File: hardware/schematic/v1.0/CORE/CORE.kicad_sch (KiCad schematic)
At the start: 80 parts, among them J1 Conn_01x06_Socket, J10 USB_C_Receptacle_USB2.0_16P, J11 Conn_01x06_Socket, J12 Conn_Coaxial, J13 Conn_01x04_Socket, J14 Conn_01x03_Socket, J15 Conn_01x05_Socket, J16 Conn_01x04_Socket, J2 Conn_Coaxial, J26 Conn_01x04_Socket, J3 Conn_Coaxial, J4 Conn_Coaxial, J5 Conn_Coaxial, J6 Conn_Coaxial, J7 Conn_Coaxial, J8 Conn_Coaxial, J9 Conn_Coaxial, M1 ZYNQ7010&7020, U1 TXS02612RTWR, U2 TPS78633, U3 SD_Card, U5 AMS1117-1.8, U6 CH340E

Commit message: sch update
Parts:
- added RGB TFTLCD1: RGBLCD, AD:FPC-TOP40, symbol Counter:FPC-40
- added U7: FPC-6P, symbol Counter:FPC-6P
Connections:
- net +3.3V: now also RGB TFTLCD1.4, U7.2
- net GND: now also RGB TFTLCD1.29, RGB TFTLCD1.3, RGB TFTLCD1.36, RGB TFTLCD1.A, RGB TFTLCD1.B, U7.3, U7.7 (SH), U7.8 (SH)
- net I2C_SCL renamed PS_I2C_SCL
- net I2C_SDA renamed PS_I2C_SDA
- net SPI1_MISO renamed PS_SPI1_MISO
- net SPI1_MOSI renamed PS_SPI1_MOSI
- net SPI1_SCLK renamed PS_SPI1_SCLK
- net SPI1_SS0 renamed PS_SPI1_SS0
- new net CTP_INT: U7.4
- new net CTP_RST: U7.1
- new net CTP_SCL: U7.6
- new net CTP_SDA: U7.5
- new net LCD_B0: RGB TFTLCD1.21
- new net LCD_B1: RGB TFTLCD1.22
- new net LCD_B2: RGB TFTLCD1.23
- new net LCD_B3: RGB TFTLCD1.24
- new net LCD_B4: RGB TFTLCD1.25
- new net LCD_B5: RGB TFTLCD1.26
- new net LCD_B6: RGB TFTLCD1.27
- new net LCD_B7: RGB TFTLCD1.28
- new net LCD_CLK: RGB TFTLCD1.30
- new net LCD_DE: RGB TFTLCD1.34
- new net LCD_DISP: RGB TFTLCD1.31
- new net LCD_G0: RGB TFTLCD1.13
- new net LCD_G1: RGB TFTLCD1.14
- new net LCD_G2: RGB TFTLCD1.15
- new net LCD_G3: RGB TFTLCD1.16
- new net LCD_G4: RGB TFTLCD1.17
- new net LCD_G5: RGB TFTLCD1.18
- new net LCD_G6: RGB TFTLCD1.19
- new net LCD_G7: RGB TFTLCD1.20
- new net LCD_HSYNC: RGB TFTLCD1.32
- new net LCD_R0: RGB TFTLCD1.5
- new net LCD_R1: RGB TFTLCD1.6
- new net LCD_R2: RGB TFTLCD1.7
- new net LCD_R3: RGB TFTLCD1.8
- new net LCD_R4: RGB TFTLCD1.9
- new net LCD_R5: RGB TFTLCD1.10
- new net LCD_R6: RGB TFTLCD1.11
- new net LCD_R7: RGB TFTLCD1.12
- new net LCD_VSYNC: RGB TFTLCD1.33
- no-connect marks 23 -> 28
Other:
- note added: "RGB888"
- moved on the sheet: J1, J11

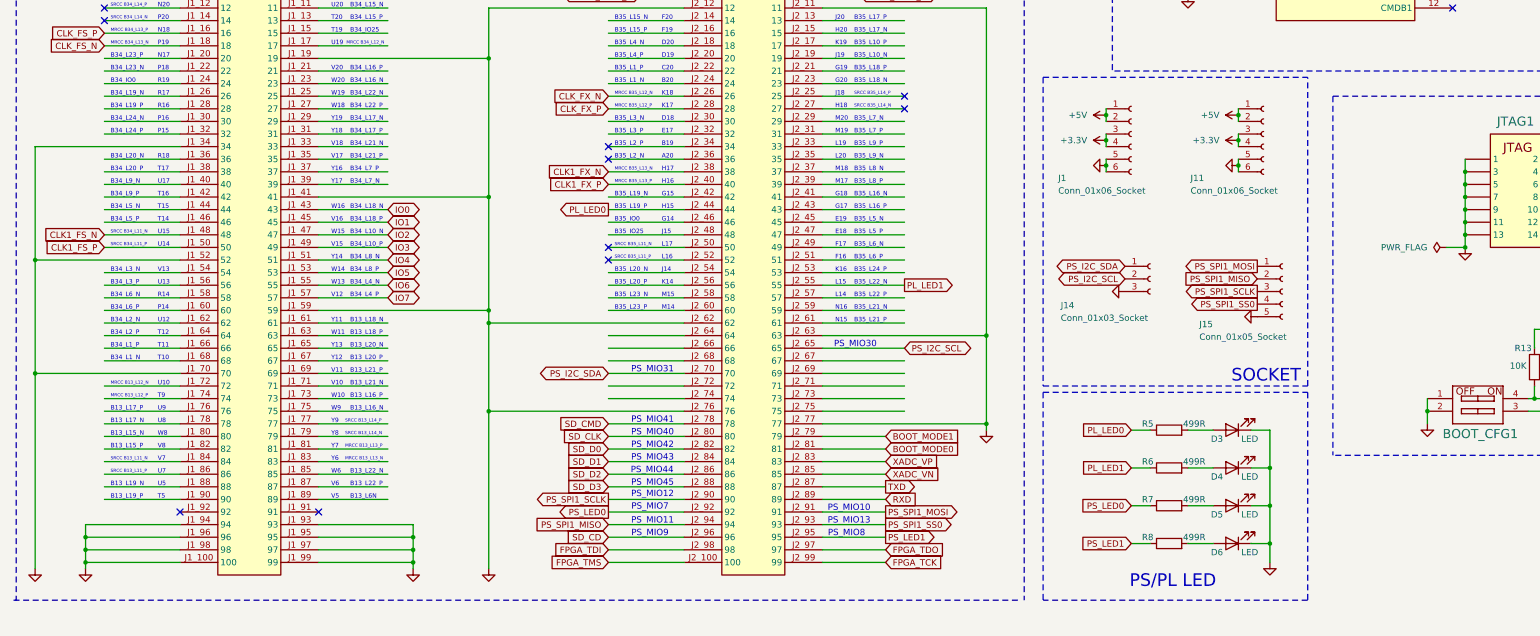
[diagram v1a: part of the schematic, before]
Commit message: sch update
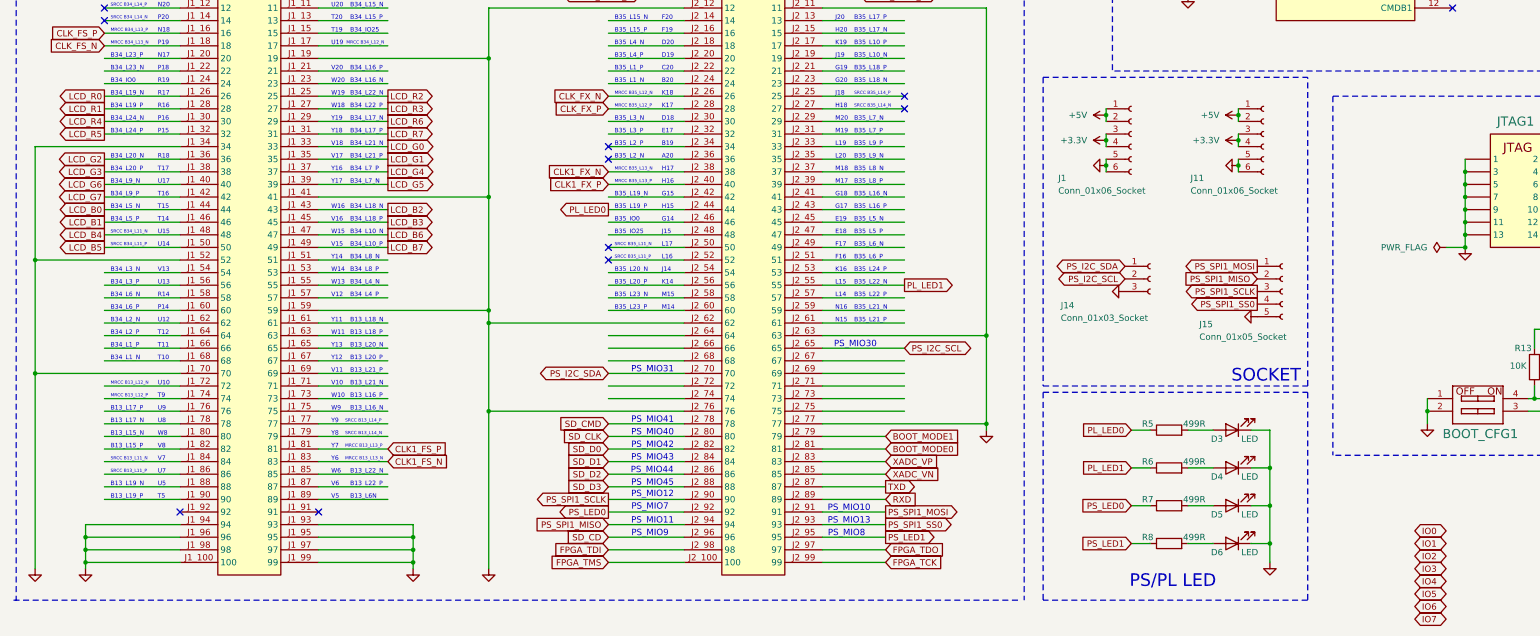
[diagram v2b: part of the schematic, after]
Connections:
- net CLK1_FS_N: now also M1.J1_83 (83); no longer M1.J1_48 (48)
- net CLK1_FS_P: now also M1.J1_81 (81); no longer M1.J1_50 (50)
- net IO0: no longer M1.J1_43 (43)
- net IO1: no longer M1.J1_45 (45)
- net IO2: no longer M1.J1_47 (47)
- net IO3: no longer M1.J1_49 (49)
- net IO4: no longer M1.J1_51 (51)
- net IO5: no longer M1.J1_53 (53)
- net IO6: no longer M1.J1_55 (55)
- net IO7: no longer M1.J1_57 (57)
- net LCD_B0: now also M1.J1_44 (44)
- net LCD_B1: now also M1.J1_46 (46)
- net LCD_B2: now also M1.J1_43 (43)
- net LCD_B3: now also M1.J1_45 (45)
- net LCD_B4: now also M1.J1_48 (48)
- net LCD_B5: now also M1.J1_50 (50)
- net LCD_B6: now also M1.J1_47 (47)
- net LCD_B7: now also M1.J1_49 (49)
- net LCD_G0: now also M1.J1_33 (33)
- net LCD_G1: now also M1.J1_35 (35)
- net LCD_G2: now also M1.J1_36 (36)
- net LCD_G3: now also M1.J1_38 (38)
- net LCD_G4: now also M1.J1_37 (37)
- net LCD_G5: now also M1.J1_39 (39)
- net LCD_G6: now also M1.J1_40 (40)
- net LCD_G7: now also M1.J1_42 (42)
- net LCD_R0: now also M1.J1_26 (26)
- net LCD_R1: now also M1.J1_28 (28)
- net LCD_R2: now also M1.J1_25 (25)
- net LCD_R3: now also M1.J1_27 (27)
- net LCD_R4: now also M1.J1_30 (30)
- net LCD_R5: now also M1.J1_32 (32)
- net LCD_R6: now also M1.J1_29 (29)
- net LCD_R7: now also M1.J1_31 (31)

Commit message: sch update
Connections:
- net CTP_INT: now also M1.J1_53 (53)
- net CTP_RST: now also M1.J1_51 (51)
- net CTP_SCL: now also M1.J1_57 (57)
- net CTP_SDA: now also M1.J1_55 (55)
- net LCD_CLK: now also M1.J1_54 (54)
- net LCD_DE: now also M1.J1_62 (62)
- net LCD_DISP: now also M1.J1_56 (56)
- net LCD_HSYNC: now also M1.J1_58 (58)
- net LCD_VSYNC: now also M1.J1_60 (60)
- net LCD_LEDK: now reaches RGB TFTLCD1.1
- net LCD_LEDA: now reaches RGB TFTLCD1.2
